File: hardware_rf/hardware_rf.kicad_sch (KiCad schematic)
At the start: 50 parts, among them IC1 CC1125RHBR, J1 Conn_Coaxial, J2 Conn_01x03_Socket, SW1 SW_Push, U1 RP2350A-QFN60, U2 W25Q128JVS, Y1 Crystal_GND24, Y2 Crystal_GND24

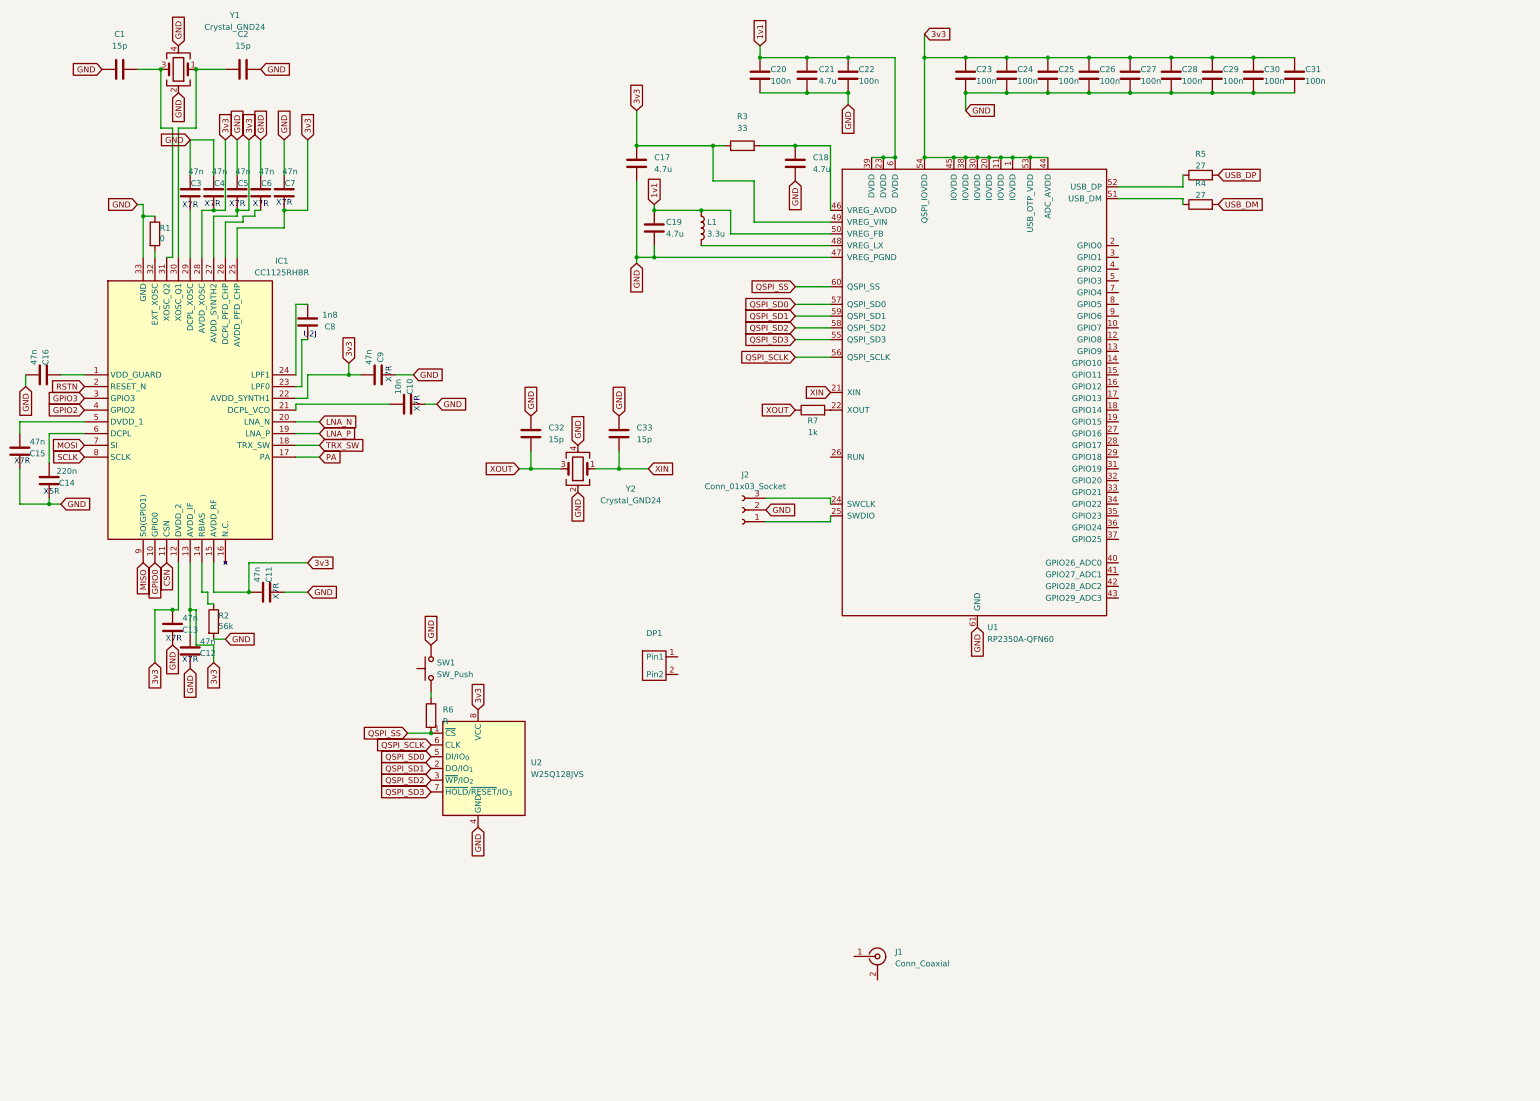
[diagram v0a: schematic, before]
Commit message: pcb
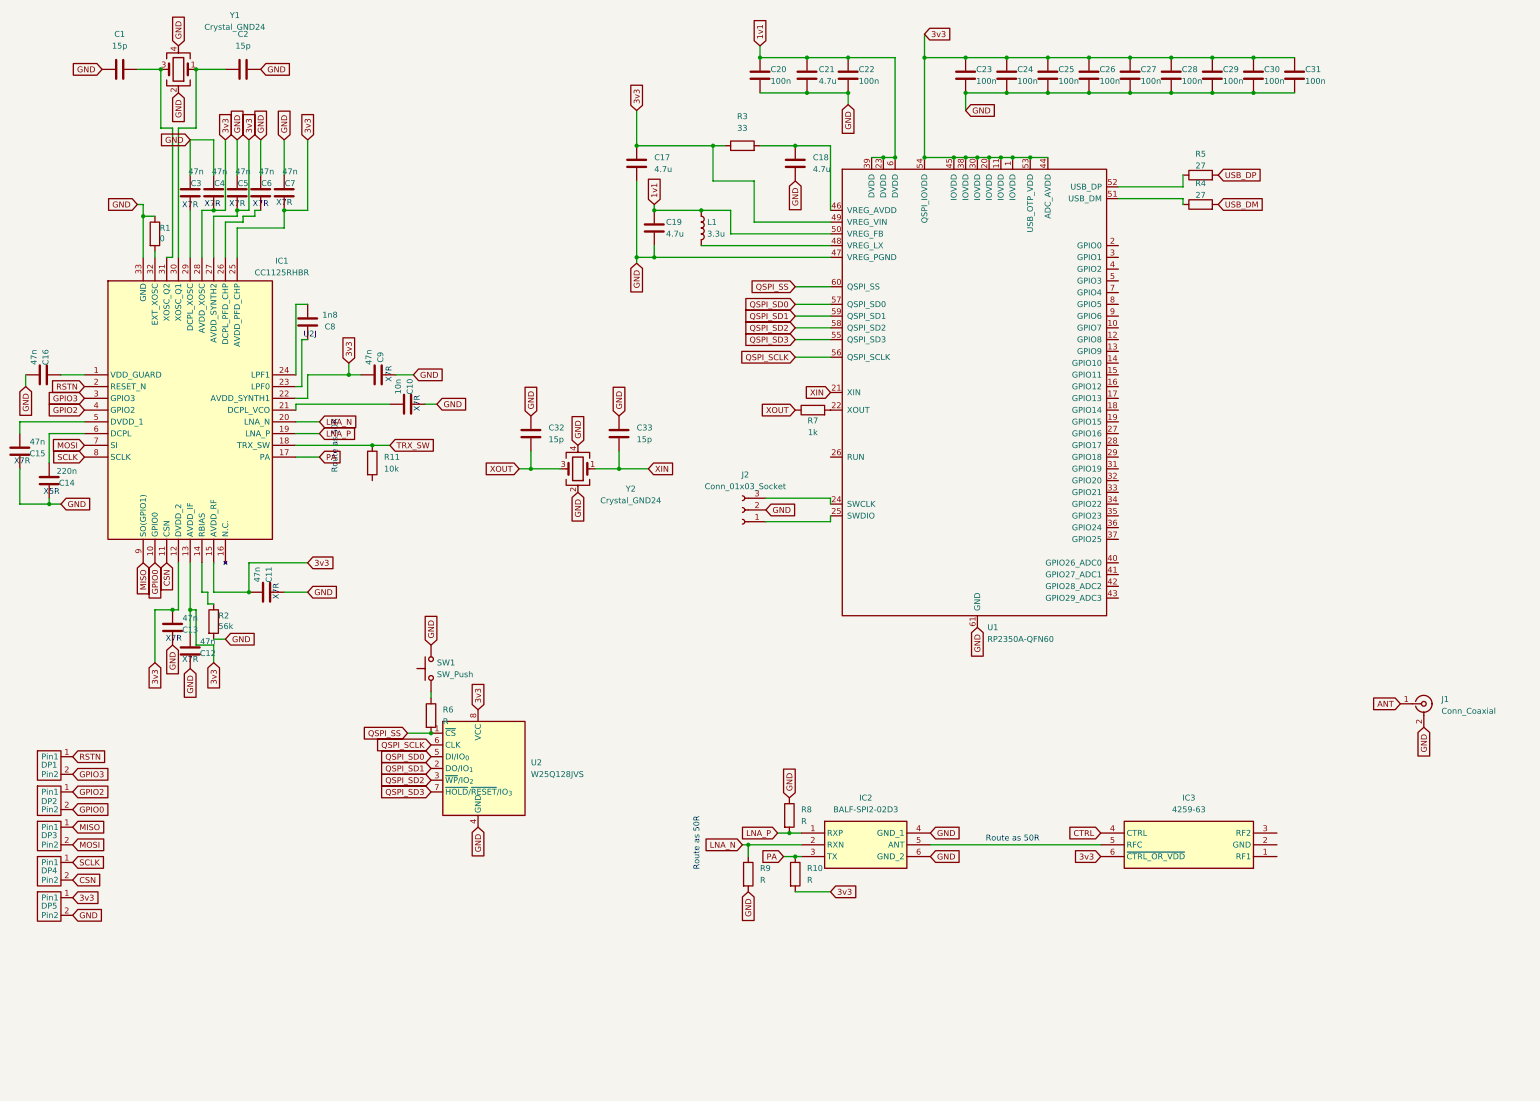
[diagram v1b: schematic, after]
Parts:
- added DP2, DP3, DP4, DP5: ~, mainfoot:Debug Pad, symbol mainlib:Debug_Pads
- added IC2: BALF-SPI2-02D3, mainfoot:BALFSPI202D3, symbol mainlib:BALF-SPI2-02D3
- added IC3: 4259-63, mainfoot:PE4259, symbol mainlib:4259-63
- added R10, R8, R9: R, symbol Device:R
- added R11: 10k, symbol Device:R
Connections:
- net 3v3: now also DP5.1 (Pin1), IC3.6 (~{CTRL_OR_VDD}), R10.2
- net CSN: now also DP4.2 (Pin2)
- net GND: now also J1.2 (Ext), DP5.2 (Pin2), IC2.4 (GND_1), IC2.6 (GND_2), R8.1, R9.2
- net GPIO0: now also DP2.2 (Pin2)
- net GPIO2: now also DP2.1 (Pin1)
- net GPIO3: now also DP1.2 (Pin2)
- net LNA_N: now also IC2.2 (RXN), R9.1
- net LNA_P: now also IC2.1 (RXP), R8.2
- net MISO: now also DP3.1 (Pin1)
- net MOSI: now also DP3.2 (Pin2)
- net PA: now also IC2.3 (TX), R10.1
- net RSTN: now also DP1.1 (Pin1)
- net SCLK: now also DP4.1 (Pin1)
- net TRX_SW: now also R11.1
- net ANT: now reaches J1.1 (In)
- new net: IC2.5 (ANT), IC3.5 (RFC)
- new net CTRL: IC3.4 (CTRL)
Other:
- note added: "Route as 50R"
- moved on the sheet: DP1, J1

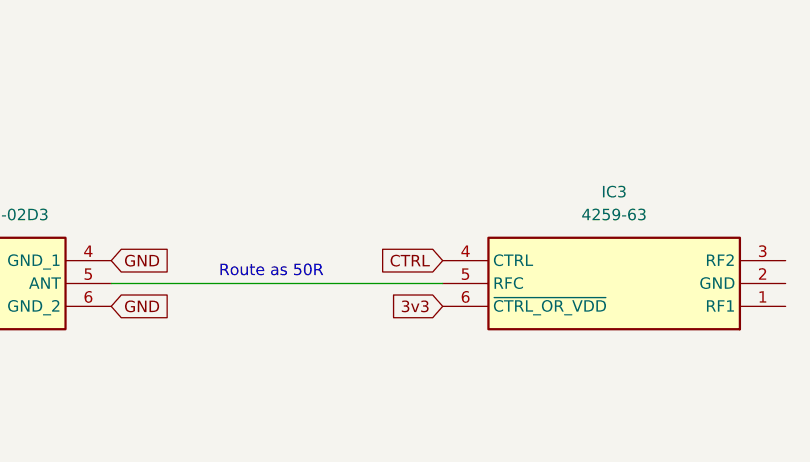
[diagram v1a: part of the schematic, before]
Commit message: pcb
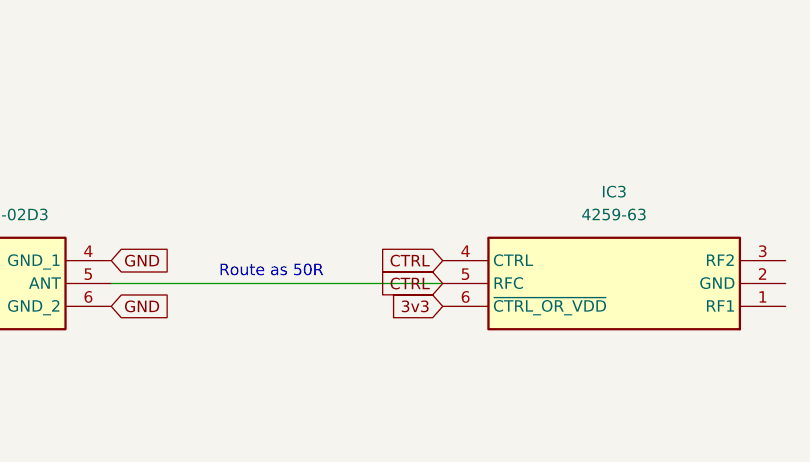
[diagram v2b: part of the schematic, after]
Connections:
- net CTRL: now also IC2.5 (ANT), IC3.5 (RFC)
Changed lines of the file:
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@@
+		)
+	)
+	(global_label "CTRL"
+		(shape input)
+		(at 255.27 210.82 180)
+		(fields_autoplaced yes)
+		(effects
+			(font
+				(size 1.27 1.27)
+			)
+			(justify right)
+		)
+		(property "Intersheetrefs" "${INTERSHEET_REFS}"
+			(at 247.7491 210.82 0)
+			(effects
+				(font
+					(size 1.27 1.27)
+				)
+				(justify right)
+				(hide yes)
+			)
 		)
 	)

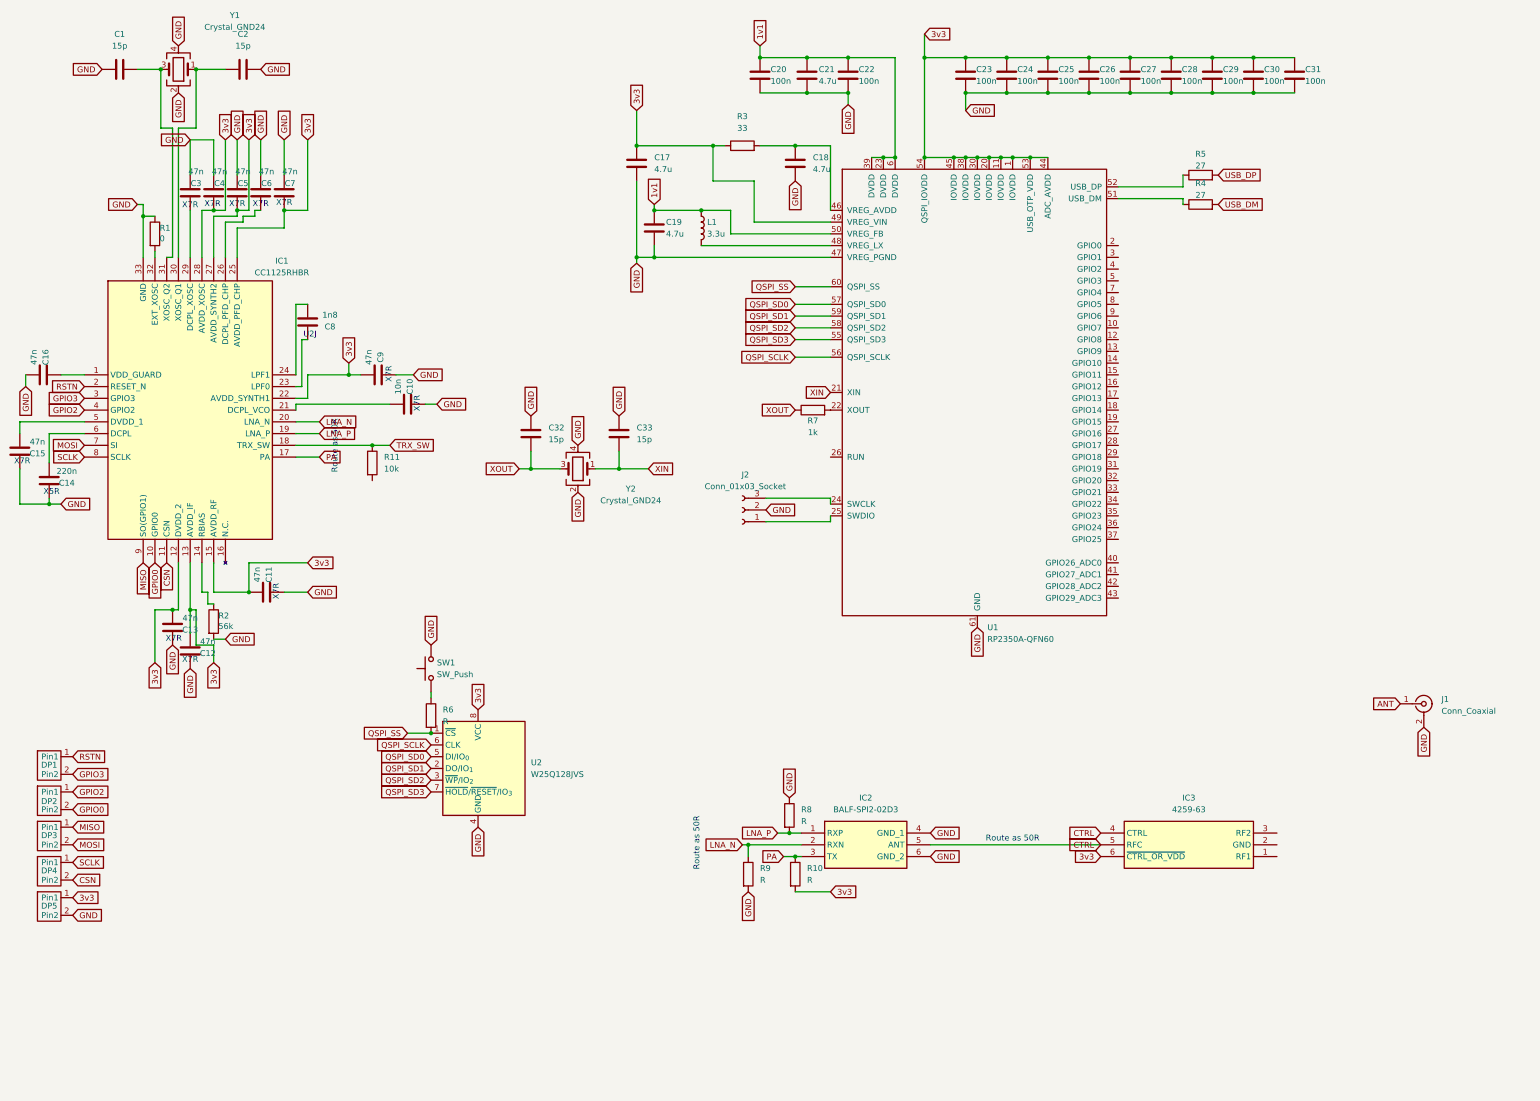
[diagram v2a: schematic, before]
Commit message: symbol
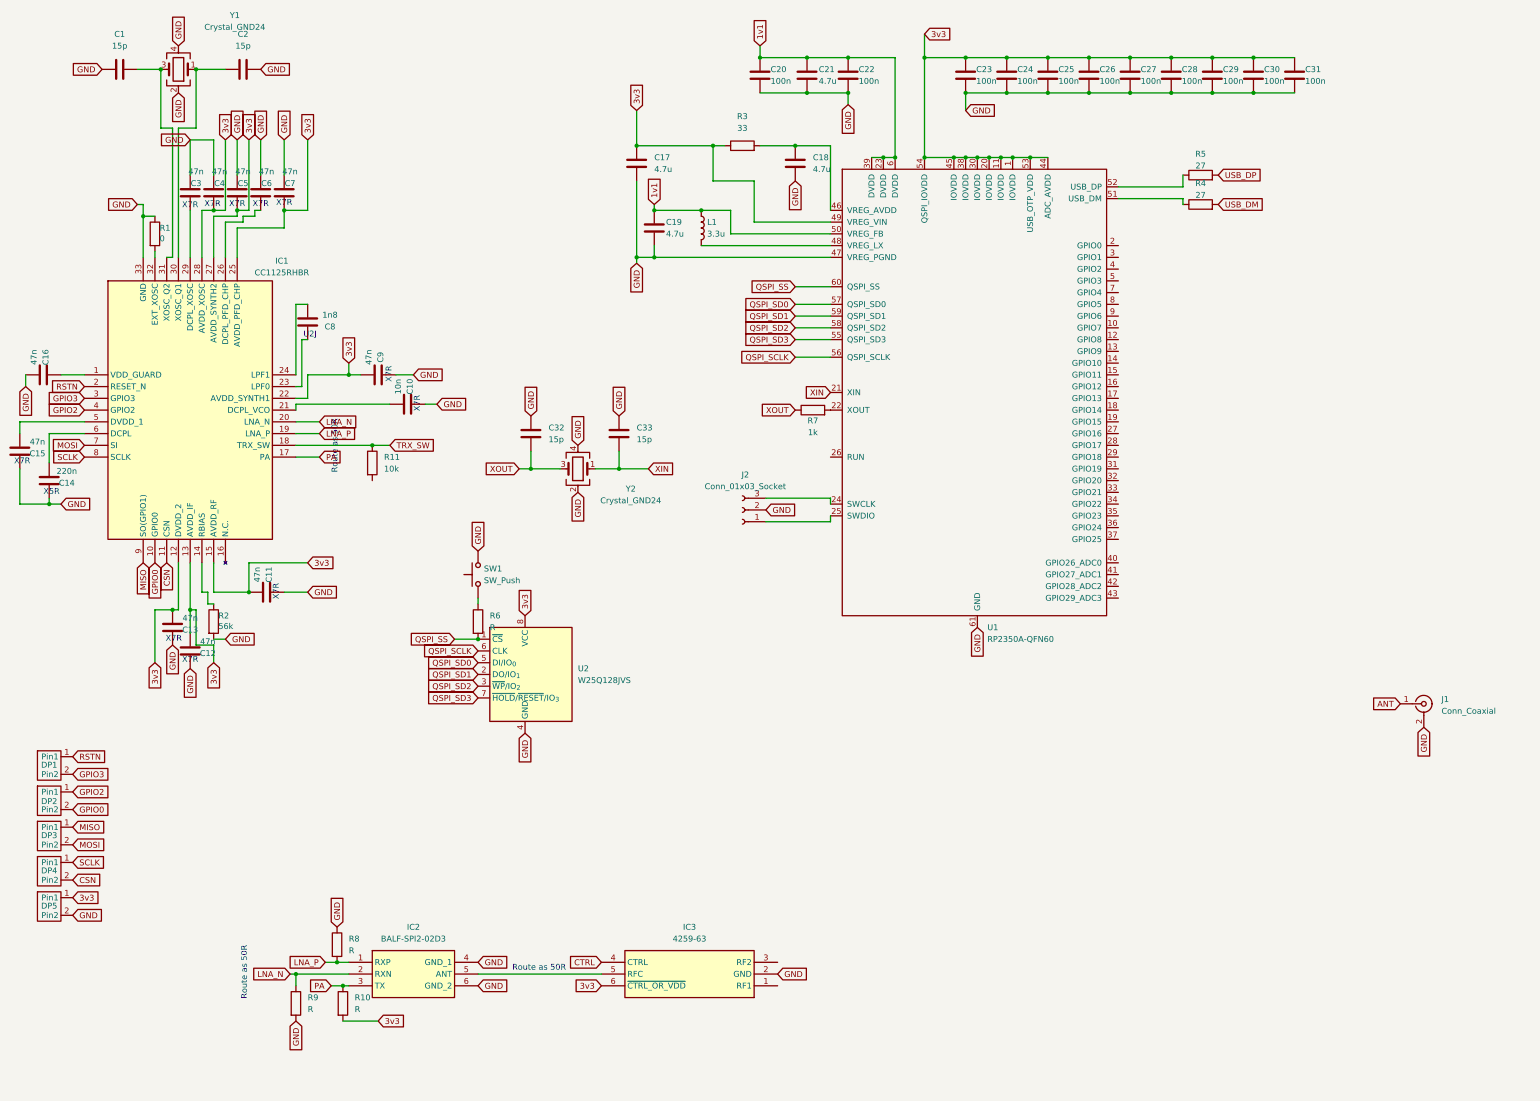
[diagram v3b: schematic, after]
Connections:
- net CTRL: no longer IC2.5 (ANT), IC3.5 (RFC)
- net GND: now also IC3.2 (GND)
- new net: IC2.5 (ANT), IC3.5 (RFC)
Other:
- moved on the sheet: IC2, IC3, R10, R6, R8, R9, SW1, U2
